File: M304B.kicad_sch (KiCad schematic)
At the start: 56 parts, among them J1 LCD 2004, J2 Relay OUT, J5 POWER IN, P1 Digital, P10 CONN_01X01, P11 CONN_01X01, P12 CONN_01X01, P13 CONN_01X01, P2 Power, P3 Analog, P4 Analog, P5 PWM, P6 PWM, P7 Communication, P8 CONN_01X01, P9 CONN_01X01, SW1 RESET, SW2 SW_A, SW3 SW_B, SW4 SW_C, SW5 SW_D, SW6 SW_ENTER, SW7 SAFEMODE, SW8 RotaryEncoder, U2 24LC256, U3 W5500, U4 LM1117-3.3, U5 74HC14

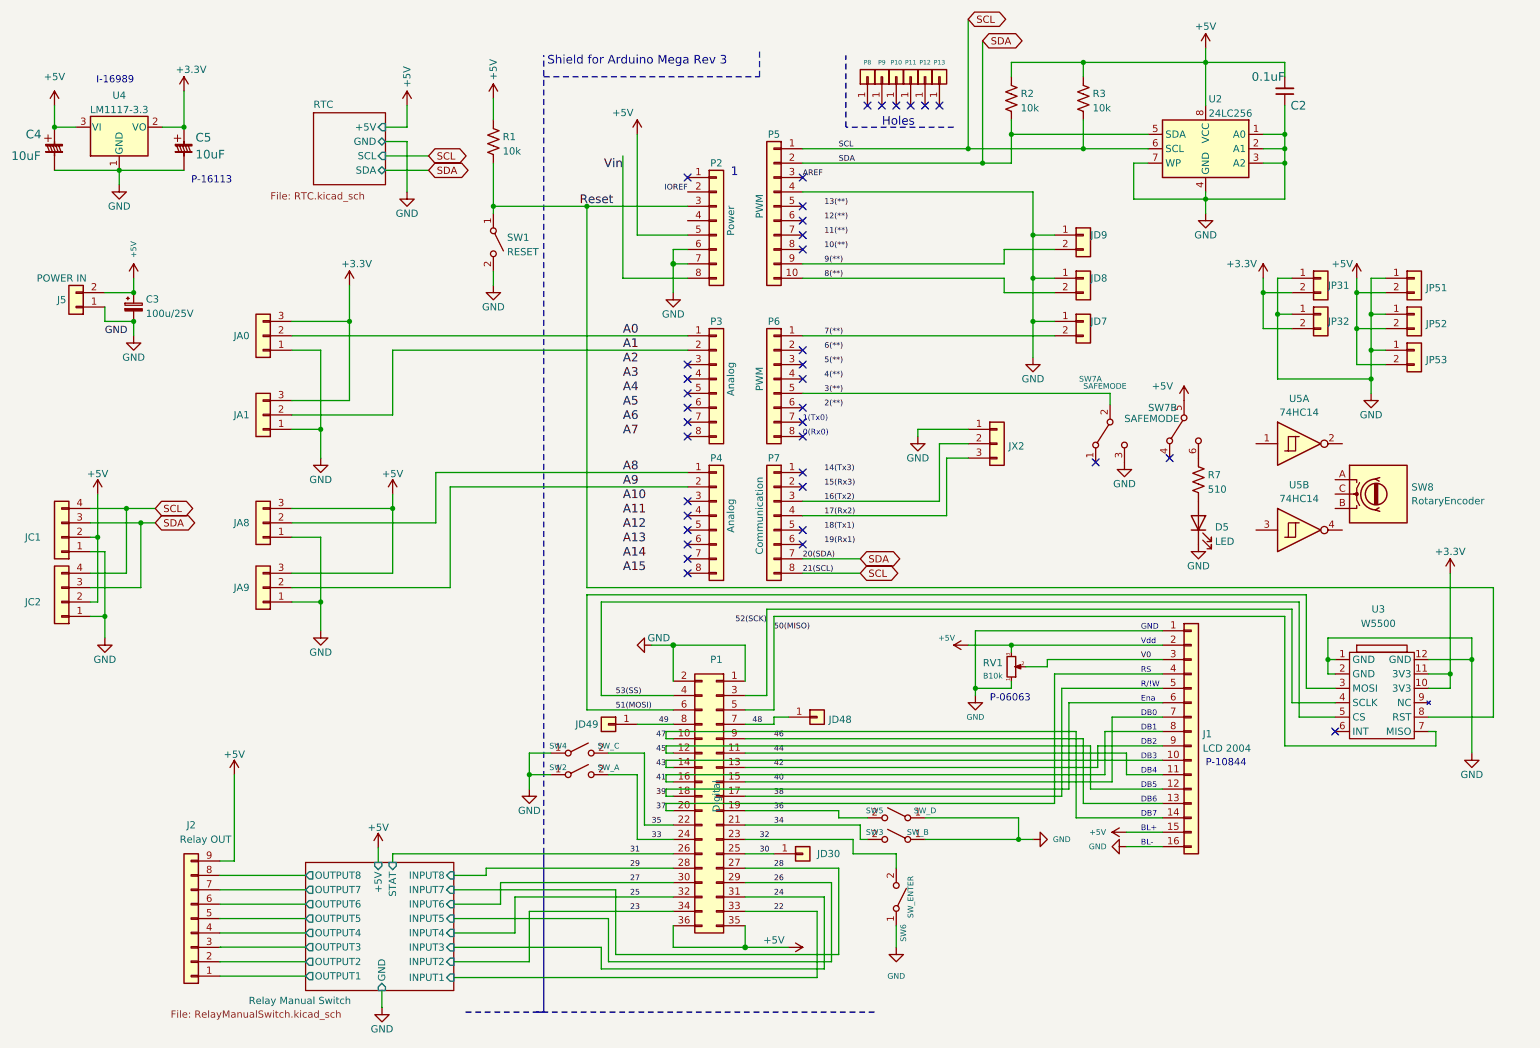
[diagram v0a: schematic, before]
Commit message: もう少し
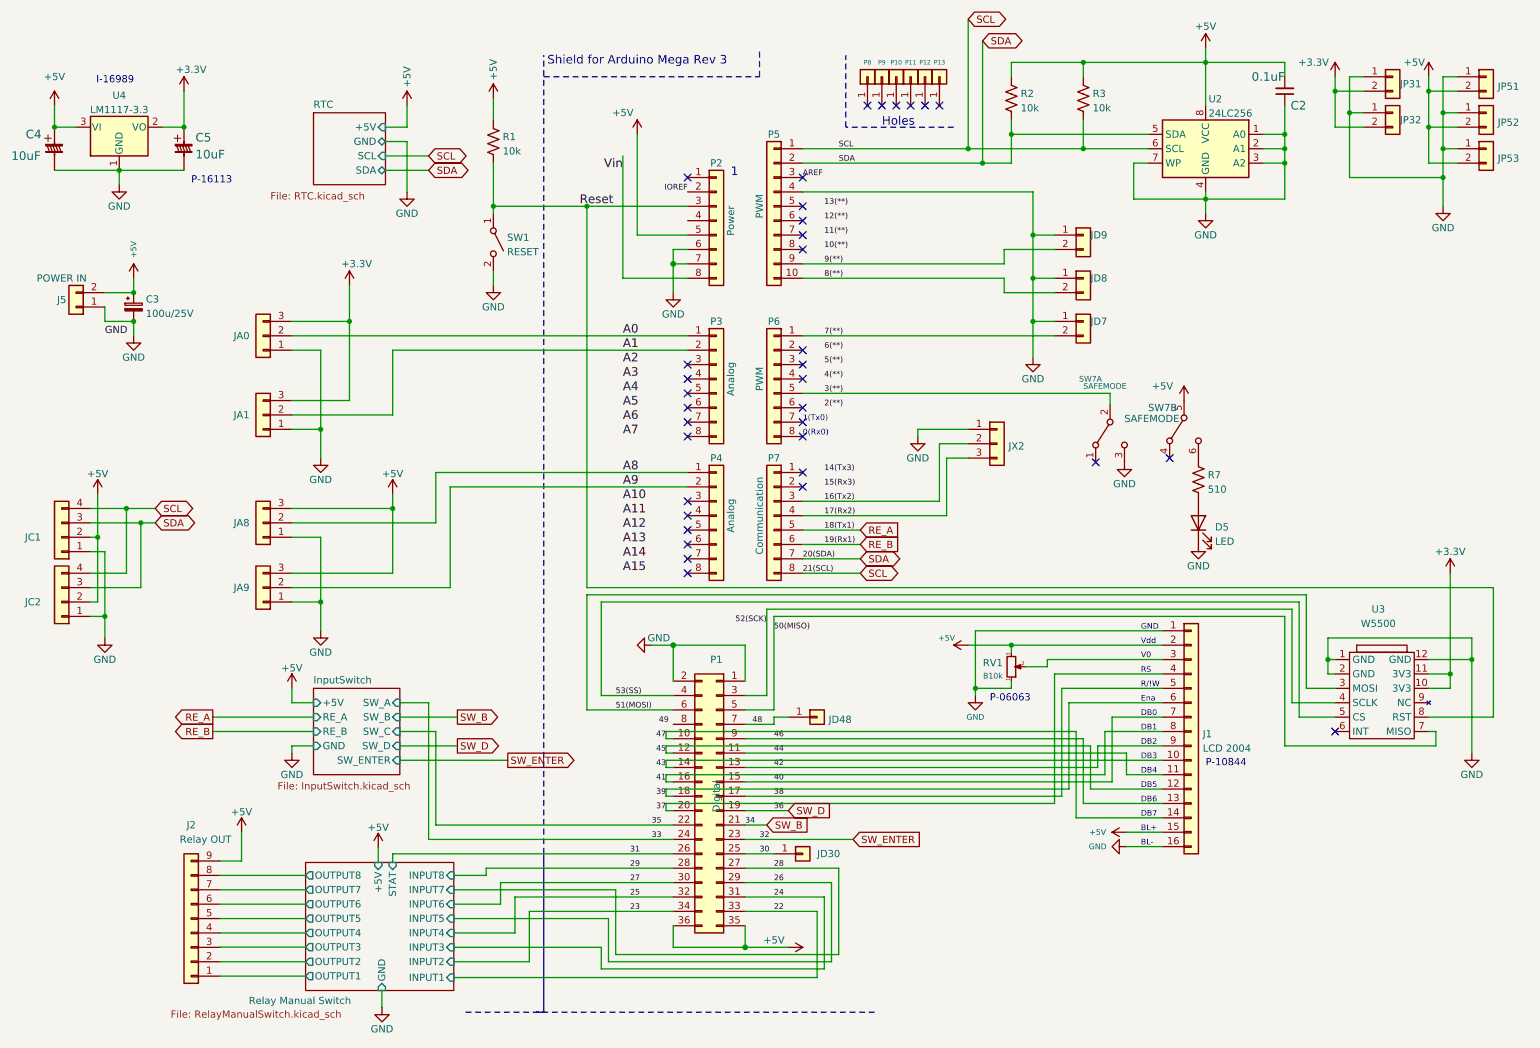
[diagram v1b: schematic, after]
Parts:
- removed JD49: Conn_01x01, Connector_Pin:Pin_D0.9mm_L10.0mm_W2.4mm_FlatFork, symbol Connector_Generic:Conn_01x01
- removed SW2: SW_A, HOLLY:TVDT18-050, symbol Switch:SW_SPST
- removed SW3: SW_B, HOLLY:TVDT18-050, symbol Switch:SW_SPST
- removed SW4: SW_C, HOLLY:TVDT18-050, symbol Switch:SW_SPST
- removed SW5: SW_D, HOLLY:TVDT18-050, symbol Switch:SW_SPST
- removed SW6: SW_ENTER, HOLLY:TVDT18-050, symbol Switch:SW_SPST
- removed SW8: RotaryEncoder, Rotary_Encoder:RotaryEncoder_Alps_EC12E_Vertical_H20mm, symbol Device:RotaryEncoder
- removed U5: 74HC14, Package_DIP:DIP-14_W7.62mm_LongPads, symbol 74xx:74HC14
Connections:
- net 49: no longer P1.8 (Pin_8)
- net RE_A: now reaches P7.5 (Pin_5)
- net RE_B: now reaches P7.6 (Pin_6)
- net 32 renamed SW_ENTER
- net 34 renamed SW_B
- net 36 renamed SW_D
- no-connect marks 37 -> 35
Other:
- added sheet InputSwitch (InputSwitch.kicad_sch)
- company: AMPSD Kyushu Univ. -> AMPSD Kyushu Univ. YS-Lab
- title: M304 UECS Controller shield for Arduino MEGA SMANOU2022 -> M304B UECS Controller shield for Arduino MEGA BABY SIZE
- moved on the sheet: JP31, JP32, JP51, JP52, JP53
